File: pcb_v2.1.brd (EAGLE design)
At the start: 19.4 x 108.4 mm, 57 parts, among them J1 PJ301_THONKICONN6, J2 PJ301_THONKICONN6, J3 PJ301_THONKICONN6, J4 PJ301_THONKICONN6, U1 MCP6004, U2 TL074_SMD, U5 TL074

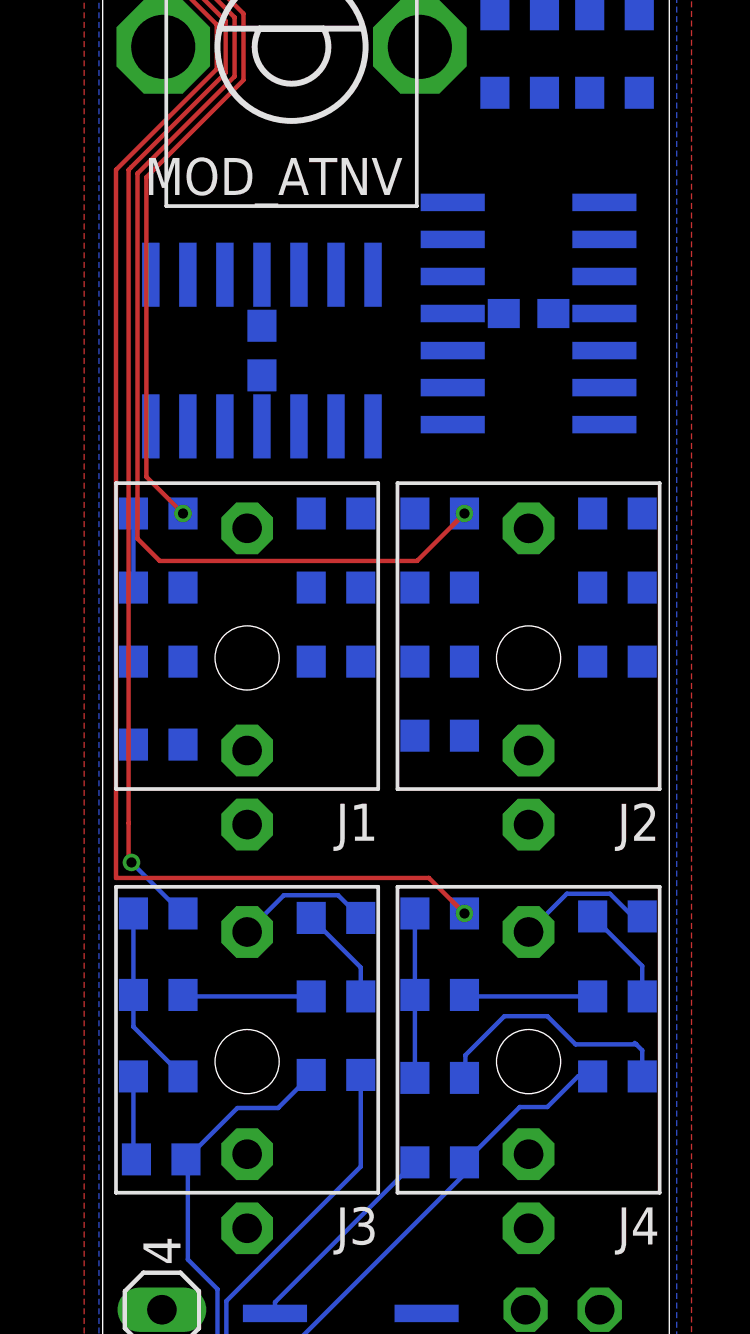
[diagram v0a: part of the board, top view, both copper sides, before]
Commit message: new board layout
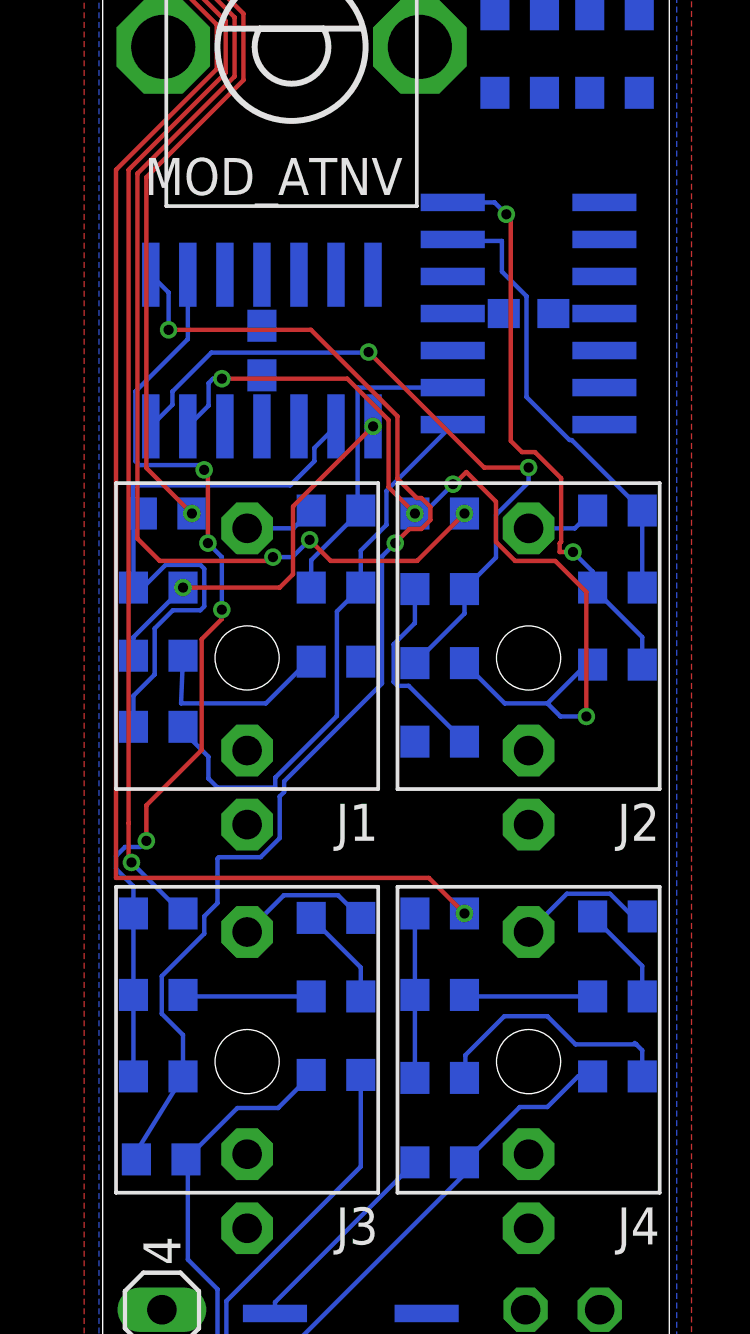
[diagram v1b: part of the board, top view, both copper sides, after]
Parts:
- moved R29 8.00 mm to (8.64, 36.9), turned to 180 degrees
- moved R31 8.00 mm to (18.3, 36.9), turned to 180 degrees
- moved R1 7.81 mm to (2.54, 32.0), turned to 180 degrees
- moved R12 6.68 mm to (12.2, 29.0)
- moved R7 6.62 mm to (12.2, 34.2)
- moved R10 6.62 mm to (12.2, 31.7)
- moved R32 6.57 mm to (18.3, 31.6)
- moved R26 6.10 mm to (18.3, 34.3)
- moved R30 0.61 mm to (2.54, 29.5)
- moved R3 0.30 mm to (2.84, 36.8)
- turned R16 to 180 degrees
- turned R2 to 180 degrees
- turned R6 to 180 degrees
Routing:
- net N$14: track 2.89 -> 43.0 mm, vias 0 -> 2
- net N$8: track 0.00 -> 32.5 mm, vias 0 -> 4
- net N$37: track 6.29 -> 32.7 mm, vias 0 -> 4
- net N$9: track 0.00 -> 24.2 mm, vias 0 -> 2
- net N$33: track 0.00 -> 20.0 mm, vias 0 -> 2
- net N$3: track 0.00 -> 19.5 mm
- net N$31: track 2.54 -> 21.6 mm
- net N$2: track 0.00 -> 15.6 mm
- net N$4: track 0.00 -> 13.2 mm, vias 0 -> 2
- net N$1: track 0.00 -> 10.9 mm
- net N$22: track 0.00 -> 6.76 mm
- net N$20: track 0.00 -> 6.69 mm
- net N$32: track 0.00 -> 2.45 mm
- net N$30: track 0.00 -> 2.45 mm
- net MID_IN: track 96.9 -> 97.5 mm, vias 1 -> 3
